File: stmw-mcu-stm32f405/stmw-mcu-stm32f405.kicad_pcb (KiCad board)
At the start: 4 copper layers, 55 x 43.5 mm, 38 parts, among them J2 TYPE-C-31-M-12, SW1 TS-1088R-02526, SW2 TS-1088R-02526, U1 AMS1117-3.3, U3 STM32F407VETx, Y1 X_16MHZ

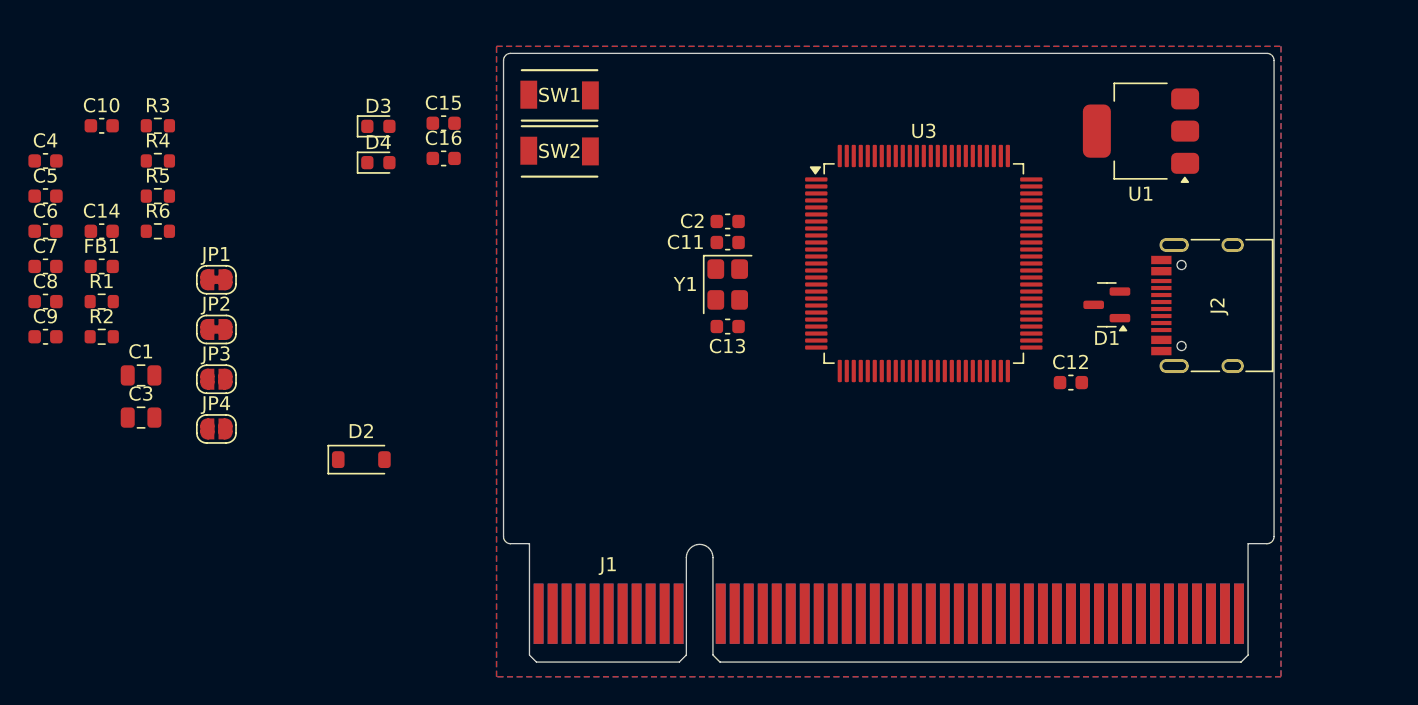
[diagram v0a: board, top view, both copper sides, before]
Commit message: Hmmmm
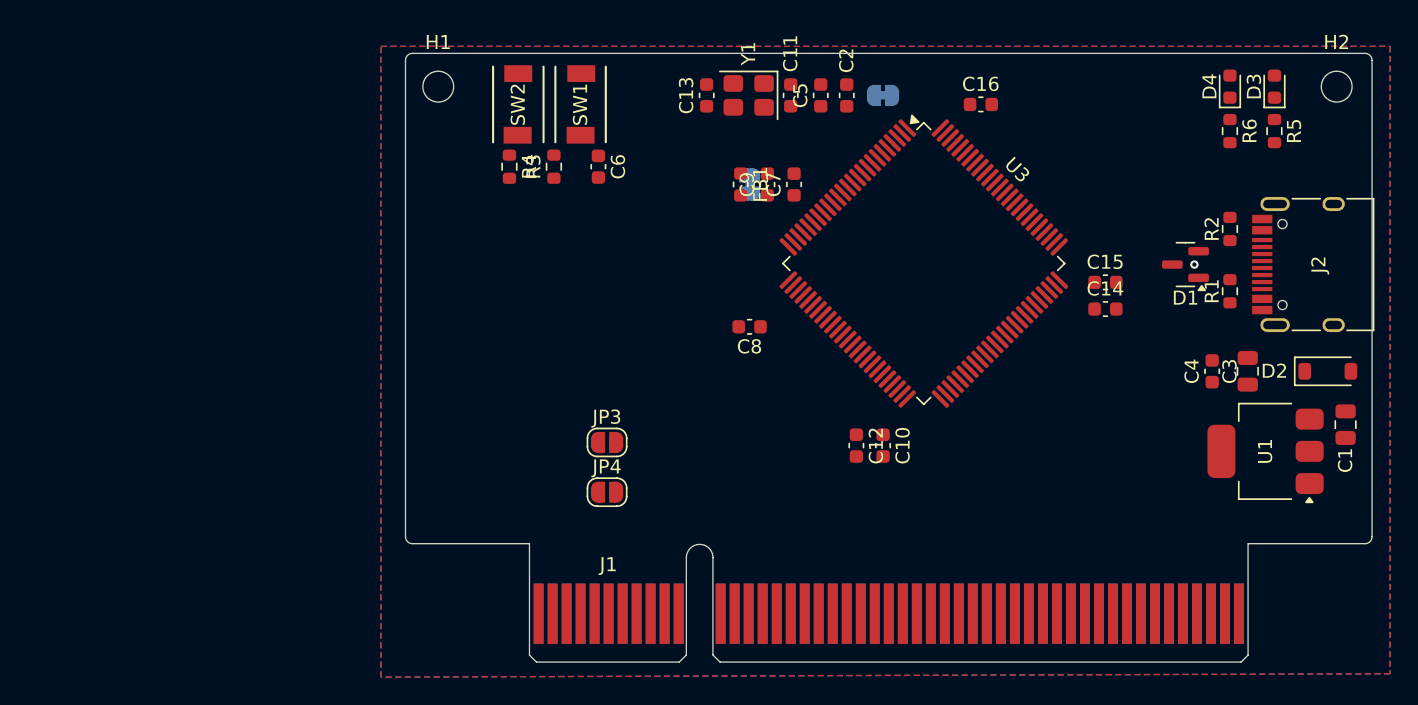
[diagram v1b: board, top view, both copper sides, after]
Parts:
- added H1: MountingHole, MountingHole:MountingHole_2.2mm_M2, F.Cu at (116.8, 79.4)
- added H2: MountingHole, MountingHole:MountingHole_2.2mm_M2, F.Cu at (181.0, 79.4)
- C12, C14: value C_2.2UF_0603 -> 2.2uF
- JP1, JP2: moved to B.Cu
- moved C1 86.1 mm to (181.6, 103.5), turned to -90 degrees
- moved C4 84.6 mm to (172.1, 99.7), turned to 90 degrees
- moved R2 80.9 mm to (173.4, 89.5), turned to -90 degrees
- moved R1 80.5 mm to (173.4, 94.0), turned to 90 degrees
- moved R5 79.8 mm to (176.5, 82.5), turned to -90 degrees
- moved C3 79.1 mm to (174.6, 99.7), turned to 90 degrees
- moved R6 76.9 mm to (173.4, 82.5), turned to -90 degrees
- moved C14 71.9 mm to (164.5, 95.2)
- moved D2 69.3 mm to (180.3, 99.7)
- moved D3 64.0 mm to (176.5, 79.4), turned to 90 degrees
- moved D4 61.0 mm to (173.4, 79.4), turned to 90 degrees
- moved C10 60.3 mm to (148.6, 105.0), turned to -90 degrees
- moved C5 55.8 mm to (144.1, 80.0), turned to 90 degrees
- moved C7 53.8 mm to (142.2, 86.4), turned to 90 degrees
- moved C9 52.7 mm to (140.3, 86.4), turned to 90 degrees
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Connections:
- J1 pad A10: unconnected-(J1-PadA10) -> PA0
- J1 pad A11: unconnected-(J1-PadA11) -> PC3
- J1 pad A12: unconnected-(J1-PadA12) -> PC2
- J1 pad A13: unconnected-(J1-PadA13) -> PC1
- J1 pad A14: unconnected-(J1-PadA14) -> PC0
- J1 pad A15: unconnected-(J1-PadA15) -> PC14
- J1 pad A16: unconnected-(J1-PadA16) -> PC13
- J1 pad A17: unconnected-(J1-PadA17) -> PE6
- J1 pad A18: unconnected-(J1-PadA18) -> PE5
- J1 pad A19: unconnected-(J1-PadA19) -> PE4
- J1 pad A20: unconnected-(J1-PadA20) -> PE3
- J1 pad A21: unconnected-(J1-PadA21) -> PE2
- J1 pad A22: unconnected-(J1-PadA22) -> PE1
- J1 pad A23: unconnected-(J1-PadA23) -> PE0
- J1 pad A24: unconnected-(J1-PadA24) -> PB9
- J1 pad A25: unconnected-(J1-PadA25) -> PB8
- J1 pad A26: unconnected-(J1-PadA26) -> PB7
- J1 pad A27: unconnected-(J1-PadA27) -> PB6
- J1 pad A28: unconnected-(J1-PadA28) -> PB5
- J1 pad A29: unconnected-(J1-PadA29) -> PB4
- J1 pad A30: unconnected-(J1-PadA30) -> PB3
- J1 pad A31: unconnected-(J1-PadA31) -> PD7
- J1 pad A32: unconnected-(J1-PadA32) -> PD6
- J1 pad A33: unconnected-(J1-PadA33) -> PD5
- J1 pad A34: unconnected-(J1-PadA34) -> PD4
- J1 pad A35: unconnected-(J1-PadA35) -> PD3
- J1 pad A36: unconnected-(J1-PadA36) -> PD2
- J1 pad A37: unconnected-(J1-PadA37) -> PD1
- J1 pad A38: unconnected-(J1-PadA38) -> PD0
- J1 pad A39: unconnected-(J1-PadA39) -> PC12
- J1 pad A40: unconnected-(J1-PadA40) -> PC11
- J1 pad A41: unconnected-(J1-PadA41) -> PC10
- J1 pad A42: unconnected-(J1-PadA42) -> PA15
- J1 pad A43: unconnected-(J1-PadA43) -> PA14
- J1 pad A8: unconnected-(J1-PadA8) -> PA2
- J1 pad A9: unconnected-(J1-PadA9) -> PA1
- J1 pad B10: (no net) -> PA5
- J1 pad B11: (no net) -> PA6
- J1 pad B12: (no net) -> PA7
- J1 pad B13: (no net) -> PC4
- J1 pad B14: (no net) -> PC5
- J1 pad B15: (no net) -> PB0
- J1 pad B16: (no net) -> PB1
- J1 pad B17: (no net) -> PB2
- J1 pad B18: (no net) -> PE7
- J1 pad B19: (no net) -> PE8
- J1 pad B20: (no net) -> PE9
- J1 pad B21: (no net) -> PE10
- J1 pad B22: (no net) -> PE11
- J1 pad B23: (no net) -> PE12
- J1 pad B24: (no net) -> PE13
- J1 pad B25: (no net) -> PE14
- J1 pad B26: (no net) -> PE15
- J1 pad B27: (no net) -> PB12
- J1 pad B28: (no net) -> PB13
- J1 pad B29: (no net) -> PB14
- J1 pad B30: (no net) -> PB15
- J1 pad B31: (no net) -> PD8
- J1 pad B32: (no net) -> PD9
- J1 pad B33: (no net) -> PD10
- J1 pad B34: (no net) -> PD11
- J1 pad B35: (no net) -> PD12
- J1 pad B36: (no net) -> PD13
- J1 pad B37: (no net) -> PD14
- J1 pad B38: (no net) -> PD15
- J1 pad B39: (no net) -> PC6
- J1 pad B4: (no net) -> unconnected-(J1-PadB4)
- J1 pad B40: (no net) -> PC7
- J1 pad B41: (no net) -> PC8
- J1 pad B42: (no net) -> PC9
- J1 pad B43: (no net) -> PA8
- J1 pad B44: (no net) -> PA9
- J1 pad B45: (no net) -> PA10
- J1 pad B46: (no net) -> PA11
- J1 pad B47: (no net) -> PA12
- J1 pad B48: (no net) -> PA13
- J1 pad B49: (no net) -> GND
- J1 pad B5: (no net) -> unconnected-(J1-PadB5)
- J1 pad B6: (no net) -> unconnected-(J1-PadB6)
- J1 pad B7: (no net) -> unconnected-(J1-PadB7)
- J1 pad B8: (no net) -> PA3
- J1 pad B9: (no net) -> PA4
- U3 pad 1: unconnected-(U3-PE2-Pad1) -> PE2
- U3 pad 15: unconnected-(U3-PC0-Pad15) -> PC0
- U3 pad 16: unconnected-(U3-PC1-Pad16) -> PC1
- U3 pad 17: unconnected-(U3-PC2-Pad17) -> PC2
- U3 pad 18: unconnected-(U3-PC3-Pad18) -> PC3
- U3 pad 2: unconnected-(U3-PE3-Pad2) -> PE3
- U3 pad 23: unconnected-(U3-PA0-Pad23) -> PA0
- U3 pad 24: unconnected-(U3-PA1-Pad24) -> PA1
- U3 pad 25: unconnected-(U3-PA2-Pad25) -> PA2
- U3 pad 26: unconnected-(U3-PA3-Pad26) -> PA3
- U3 pad 29: unconnected-(U3-PA4-Pad29) -> PA4
- U3 pad 3: unconnected-(U3-PE4-Pad3) -> PE4
- U3 pad 30: unconnected-(U3-PA5-Pad30) -> PA5
- U3 pad 31: unconnected-(U3-PA6-Pad31) -> PA6
- U3 pad 32: unconnected-(U3-PA7-Pad32) -> PA7
- U3 pad 33: unconnected-(U3-PC4-Pad33) -> PC4
- U3 pad 34: unconnected-(U3-PC5-Pad34) -> PC5
- U3 pad 35: unconnected-(U3-PB0-Pad35) -> PB0
- U3 pad 36: unconnected-(U3-PB1-Pad36) -> PB1
- U3 pad 37: unconnected-(U3-PB2-Pad37) -> PB2
- U3 pad 38: unconnected-(U3-PE7-Pad38) -> PE7
- U3 pad 39: unconnected-(U3-PE8-Pad39) -> PE8
- U3 pad 4: unconnected-(U3-PE5-Pad4) -> PE5
- U3 pad 40: unconnected-(U3-PE9-Pad40) -> PE9
- U3 pad 41: unconnected-(U3-PE10-Pad41) -> PE10
- U3 pad 42: unconnected-(U3-PE11-Pad42) -> PE11
- U3 pad 43: unconnected-(U3-PE12-Pad43) -> PE12
- U3 pad 44: unconnected-(U3-PE13-Pad44) -> PE13
- U3 pad 45: unconnected-(U3-PE14-Pad45) -> PE14
- U3 pad 46: unconnected-(U3-PE15-Pad46) -> PE15
- U3 pad 47: unconnected-(U3-PB10-Pad47) -> PB10
- U3 pad 48: unconnected-(U3-PB11-Pad48) -> PB11
- U3 pad 5: unconnected-(U3-PE6-Pad5) -> PE6
- U3 pad 51: unconnected-(U3-PB12-Pad51) -> PB12
- U3 pad 52: unconnected-(U3-PB13-Pad52) -> PB13
- U3 pad 53: unconnected-(U3-PB14-Pad53) -> PB14
- U3 pad 54: unconnected-(U3-PB15-Pad54) -> PB15
- U3 pad 55: unconnected-(U3-PD8-Pad55) -> PD8
- U3 pad 56: unconnected-(U3-PD9-Pad56) -> PD9
- U3 pad 57: unconnected-(U3-PD10-Pad57) -> PD10
- U3 pad 58: unconnected-(U3-PD11-Pad58) -> PD11
- U3 pad 59: unconnected-(U3-PD12-Pad59) -> PD12
- U3 pad 60: unconnected-(U3-PD13-Pad60) -> PD13
- U3 pad 61: unconnected-(U3-PD14-Pad61) -> PD14
- U3 pad 62: unconnected-(U3-PD15-Pad62) -> PD15
- U3 pad 63: unconnected-(U3-PC6-Pad63) -> PC6
- U3 pad 64: unconnected-(U3-PC7-Pad64) -> PC7
- U3 pad 65: unconnected-(U3-PC8-Pad65) -> PC8
- U3 pad 66: unconnected-(U3-PC9-Pad66) -> PC9
- U3 pad 67: unconnected-(U3-PA8-Pad67) -> PA8
- U3 pad 68: unconnected-(U3-PA9-Pad68) -> PA9
- U3 pad 69: unconnected-(U3-PA10-Pad69) -> PA10
- U3 pad 7: unconnected-(U3-PC13-Pad7) -> PC13
- U3 pad 72: unconnected-(U3-PA13-Pad72) -> PA13
- U3 pad 76: unconnected-(U3-PA14-Pad76) -> PA14
- U3 pad 77: unconnected-(U3-PA15-Pad77) -> PA15
- U3 pad 78: unconnected-(U3-PC10-Pad78) -> PC10
- U3 pad 79: unconnected-(U3-PC11-Pad79) -> PC11
- U3 pad 8: unconnected-(U3-PC14-Pad8) -> PC14
- U3 pad 80: unconnected-(U3-PC12-Pad80) -> PC12
- U3 pad 81: unconnected-(U3-PD0-Pad81) -> PD0
- U3 pad 82: unconnected-(U3-PD1-Pad82) -> PD1
- U3 pad 83: unconnected-(U3-PD2-Pad83) -> PD2
- U3 pad 84: unconnected-(U3-PD3-Pad84) -> PD3
- U3 pad 85: unconnected-(U3-PD4-Pad85) -> PD4
- U3 pad 86: unconnected-(U3-PD5-Pad86) -> PD5
- U3 pad 87: unconnected-(U3-PD6-Pad87) -> PD6
- U3 pad 88: unconnected-(U3-PD7-Pad88) -> PD7
- U3 pad 89: unconnected-(U3-PB3-Pad89) -> PB3
- U3 pad 9: unconnected-(U3-PC15-Pad9) -> BO0
- U3 pad 90: unconnected-(U3-PB4-Pad90) -> PB4
- U3 pad 91: unconnected-(U3-PB5-Pad91) -> PB5
- U3 pad 92: unconnected-(U3-PB6-Pad92) -> PB6
- U3 pad 93: unconnected-(U3-PB7-Pad93) -> PB7
- U3 pad 95: unconnected-(U3-PB8-Pad95) -> PB8
- U3 pad 96: unconnected-(U3-PB9-Pad96) -> PB9
- U3 pad 97: unconnected-(U3-PE0-Pad97) -> PE0
- U3 pad 98: unconnected-(U3-PE1-Pad98) -> PE1
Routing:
- net GND: vias 0 -> 1
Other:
- board size 55 x 43.5 mm -> 69 x 43.5 mm
